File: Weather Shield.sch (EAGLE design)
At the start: 46 parts, among them J1 GP-635T, Q1 BSS138, Q2 BSS138, U1 ARDUINO_R3_SHIELD, U2 3.3V MIC5219, U3 ALS-PT19, U4 MPL3115A2LGA8, U5 HTU21D

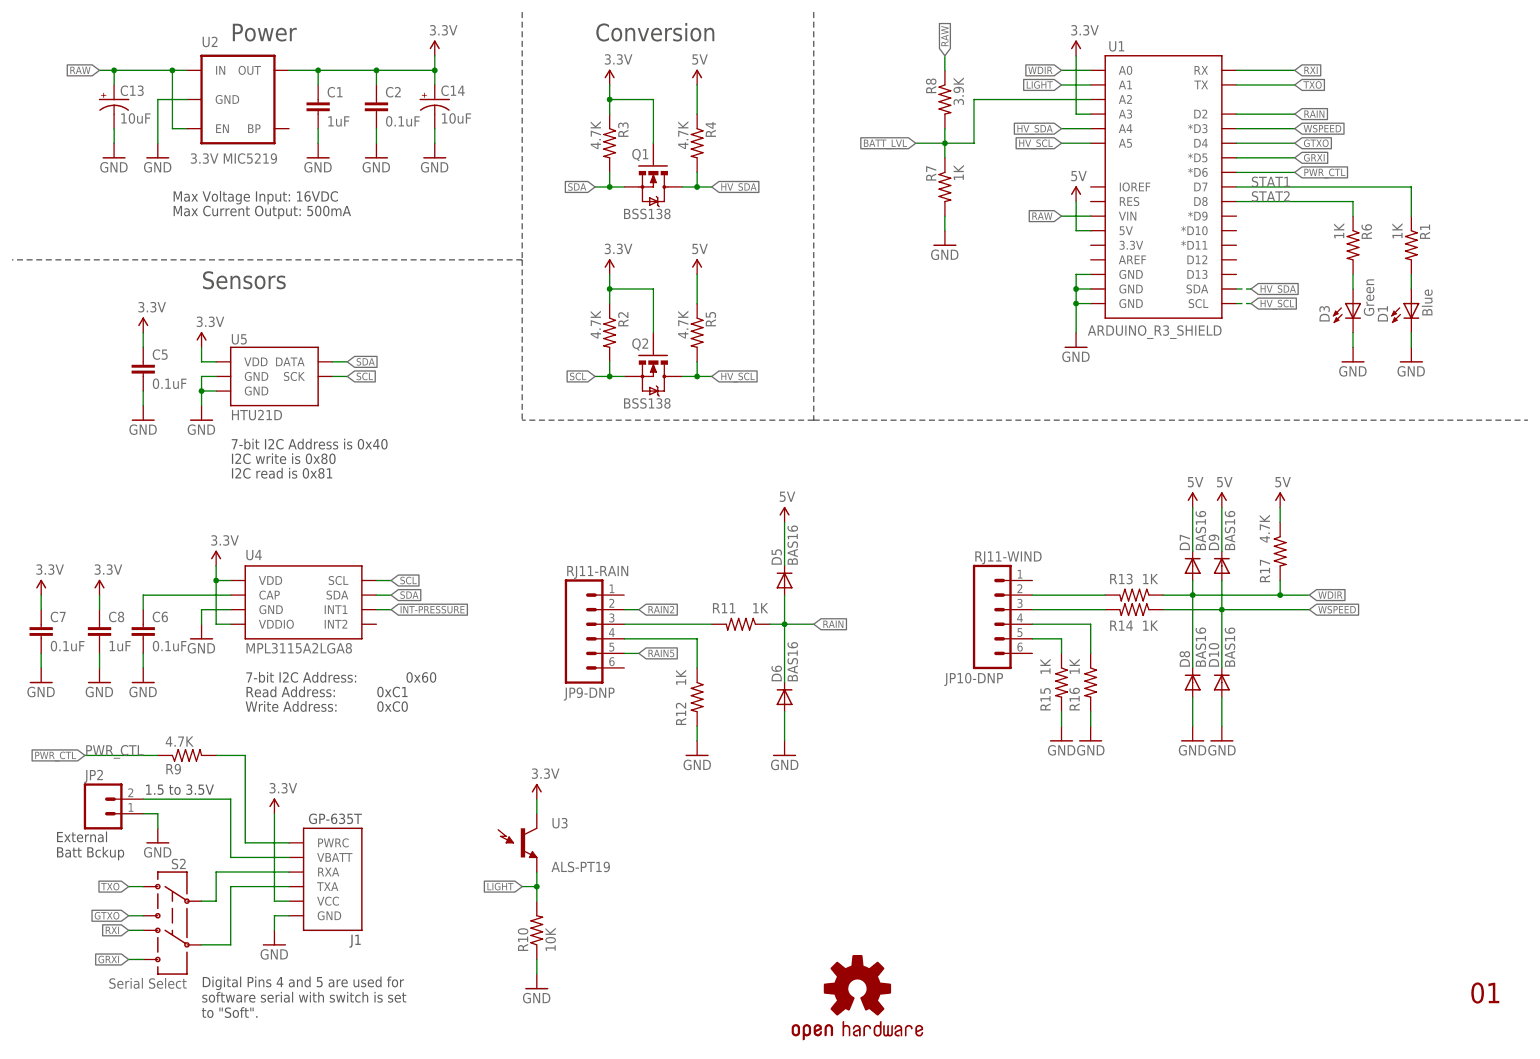
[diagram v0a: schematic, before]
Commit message: Initial commit
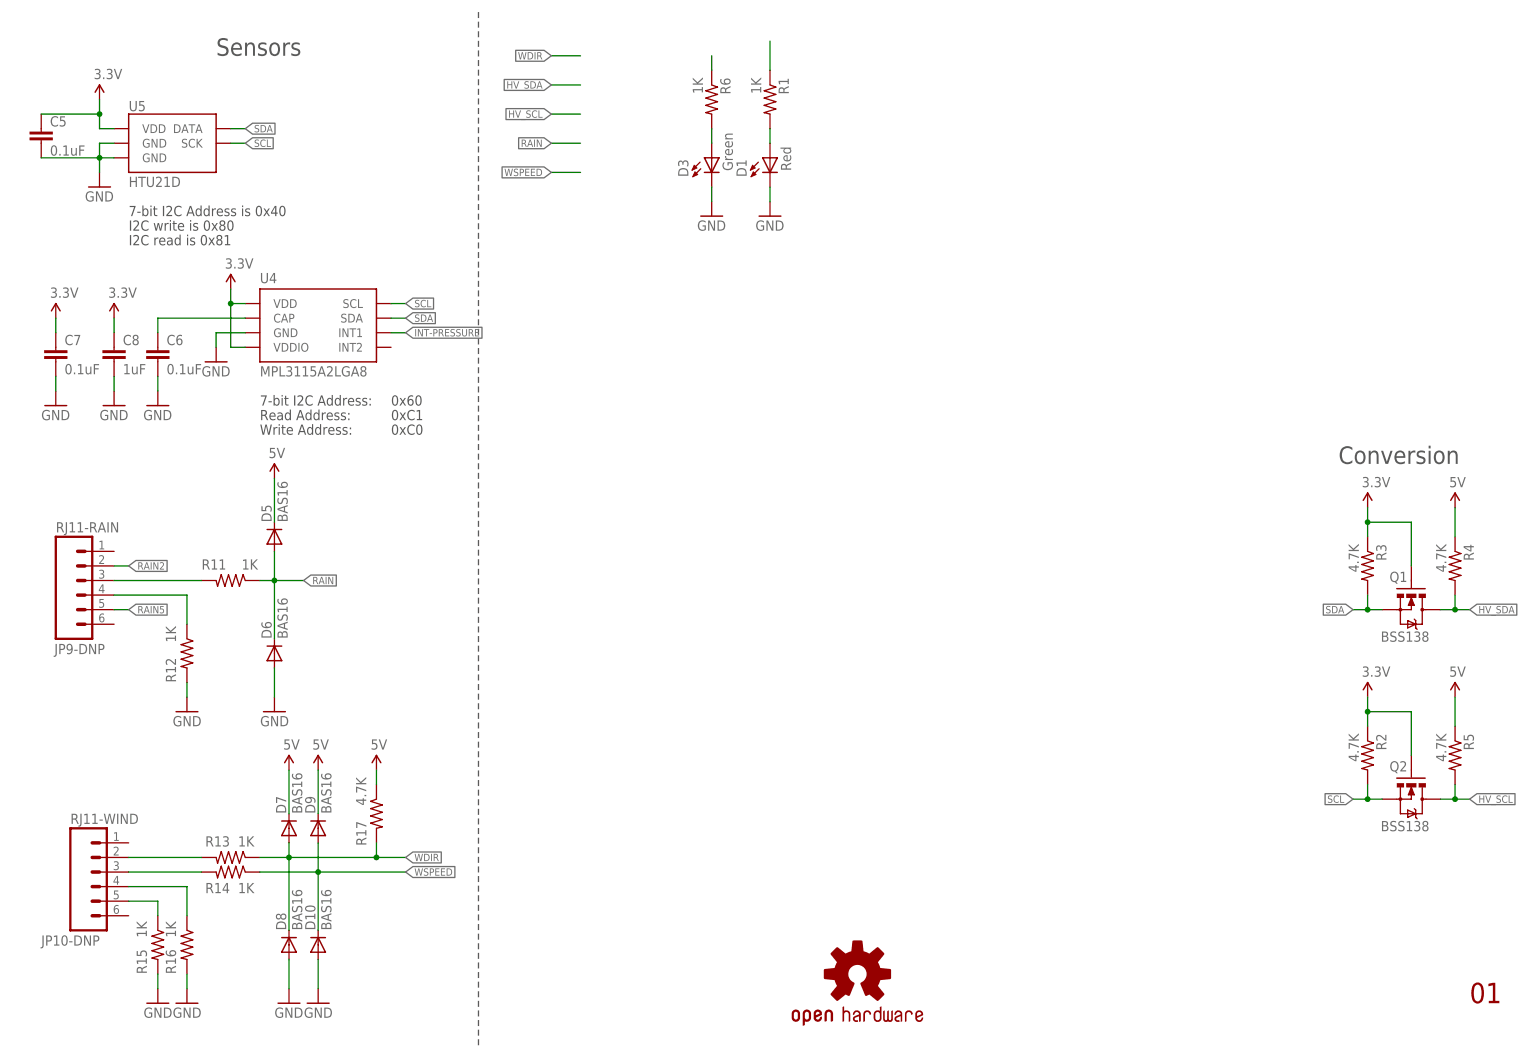
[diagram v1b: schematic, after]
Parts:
- removed C1: 1uF, SparkFun:CAP0603-CAP
- removed C13, C14: 10uF, SparkFun-Passives:CAP_POL1206
- removed C2: 0.1uF, SparkFun:CAP0603-CAP
- removed J1: GP-635T, SparkFun-Sensors:GP-635TSMD
- removed JP2: External Batt Bckup, SparkFun-Connectors:M02PTH
- removed R10: 10K, SparkFun-Passives:RESISTOR0603-RES
- removed R7: 1K, SparkFun:RESISTOR0603-RES
- removed R8: 3.9K, SparkFun:RESISTOR0603-RES
- removed R9: 4.7K, SparkFun:RESISTOR0603-RES
- removed S2: Serial Select, SparkFun-Electromechanical:SWITCH-DPDTAYZ0202
- removed U1: ARDUINO_R3_SHIELD, SparkFun-Boards:ARDUINO_R3_SHIELD
- removed U2: 3.3V MIC5219, SparkFun:V_REG_LDOSMD
- removed U3: ALS-PT19, SparkFun-Sensors:LIGHTSENSORALS
- D1: value Blue -> Red
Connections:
- removed net 3V_PWR_CTL: J1.PWRC, R9.2
- removed net BATT_LVL: R7.1, R8.2, U1.A2
- removed net GPS-RX: J1.RXA, S2.2
- removed net GPS-TX: J1.TXA, S2.5
- removed net GRXI: S2.6, U1.*D5
- removed net GTXO: S2.3, U1.D4
- removed net LIGHT: R10.2, U1.A1, U3.E1
- removed net PWR_CTL: R9.1, U1.*D6
- removed net RAW: C13.+, R8.1, U1.VIN, U2.EN, U2.IN
- removed net RXI: S2.4, U1.RX
- removed net TXO: S2.1, U1.TX
- removed net V_BATT: J1.VBATT, JP2.2
- net 3.3V: no longer C1.1, C14.+, C2.1, J1.VCC, U1.A3, U2.OUT, U3.C1
- net 5V: no longer U1.5V
- net GND: no longer C1.2, C13.-, C14.-, C2.2, J1.GND, JP2.1, R10.1, R7.2, U1.GND@0, U1.GND@1, U1.GND@2, U2.GND
- net HV_SCL: no longer U1.A5, U1.SCL
- net HV_SDA: no longer U1.A4, U1.SDA
- net RAIN: no longer U1.D2
- net STAT1: no longer U1.D7
- net STAT2: no longer U1.D8
- net WDIR: no longer U1.A0
- net WSPEED: no longer U1.*D3
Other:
- note added: "Rain sensor"
- note added: "Wind Speed & Direction"
- note removed: "1.5 to 3.5V"
- note removed: "Digital Pins 4 and 5 are used for software serial with switch is set to "Soft"."
- note removed: "External Batt Bckup"
- note removed: "GPS (optional)"
- note removed: "Light"
- note removed: "Max Current Output: 500mA"
- note removed: "Max Voltage Input: 16VDC"
- note removed: "Power"
- note removed: "Rain (optional)"
- note removed: "Wind (optional)"
- moved on the sheet: C5, C6, C7, C8, D1, D10, D3, D5, D6, D7, D8, D9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
